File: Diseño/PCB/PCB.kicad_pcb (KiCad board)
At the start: 2 copper layers, 26 parts, among them J1 Bateria, P101 USB_C_Plug_USB2.0, Q101 SS8050, Q102 SS8050, U1 SDP31-500PA-TR-250PCS, U101 AMS1117-3.3, U102 CH340C, U2 SCD41-D-R2, U3 BME688

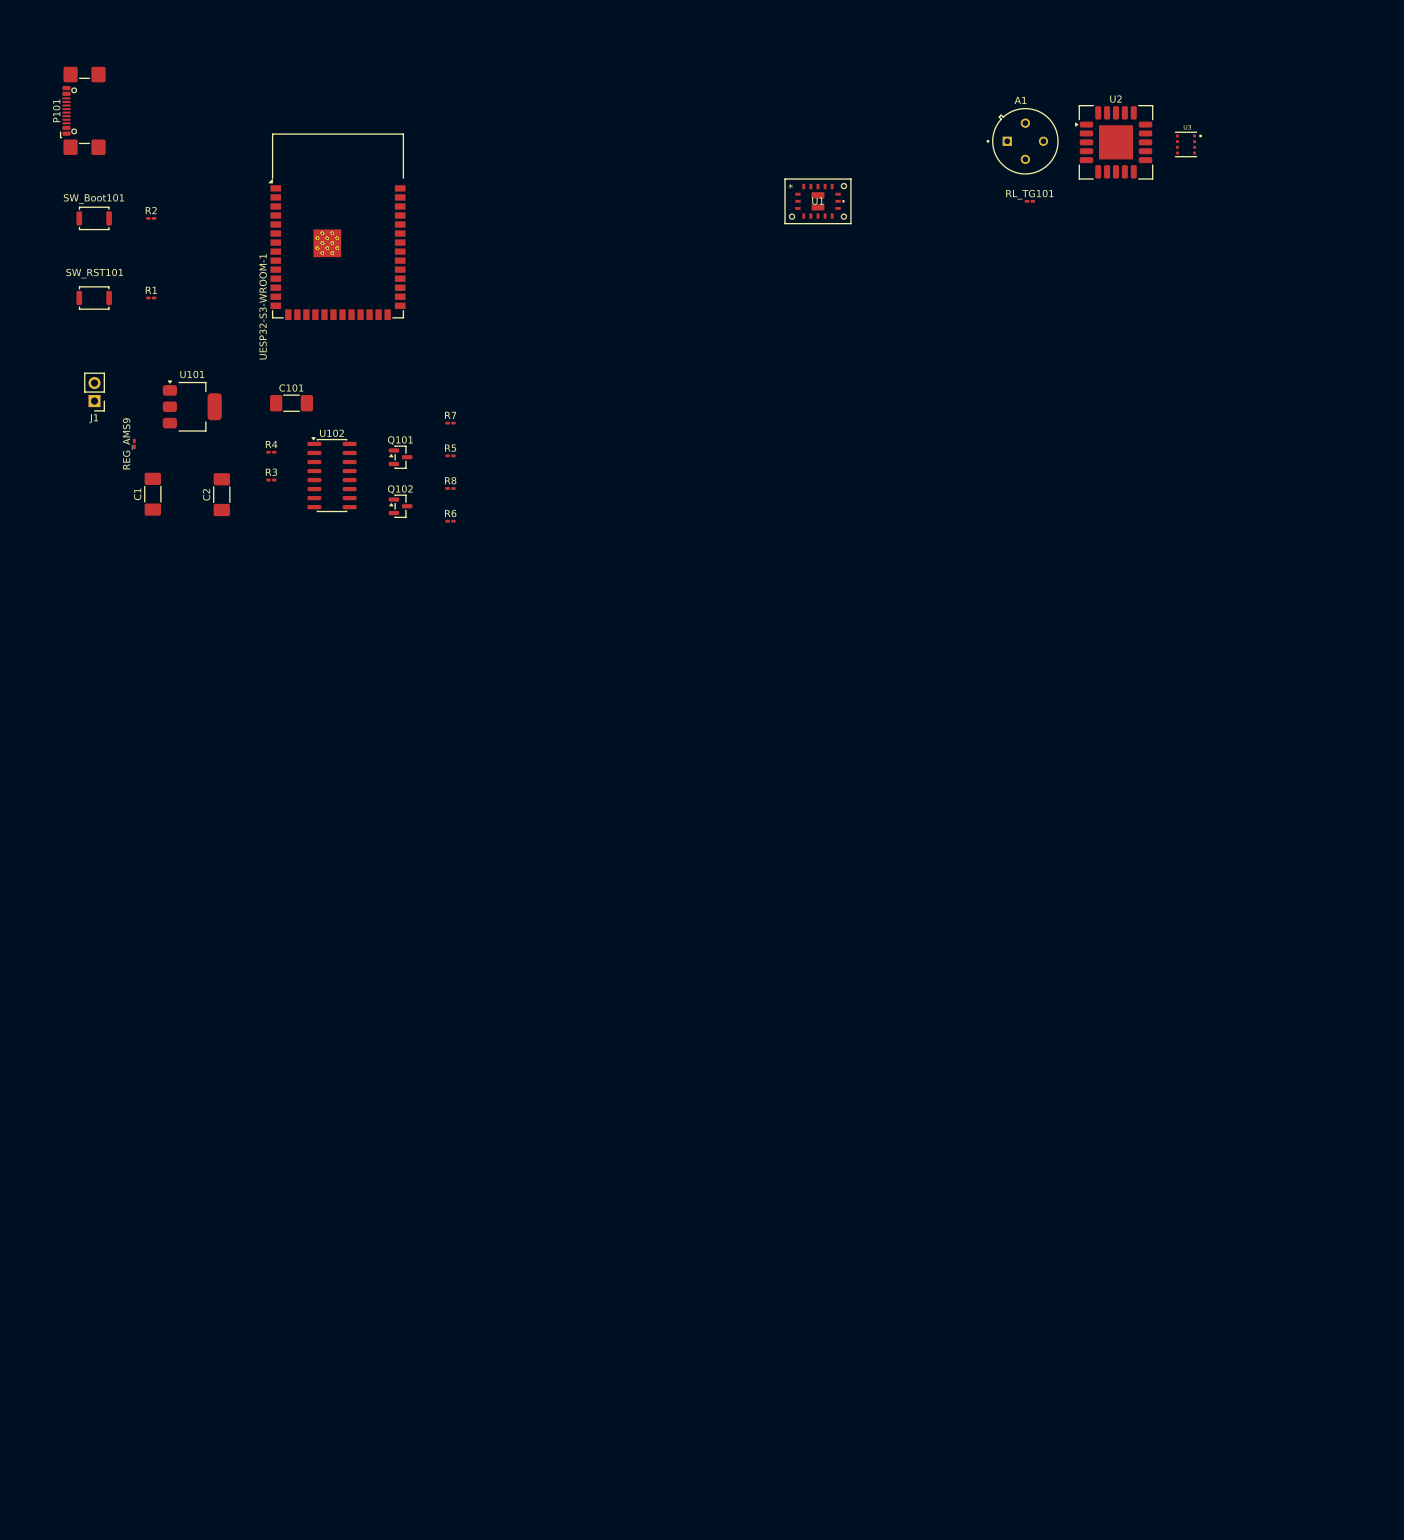
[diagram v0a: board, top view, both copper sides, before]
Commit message: Update
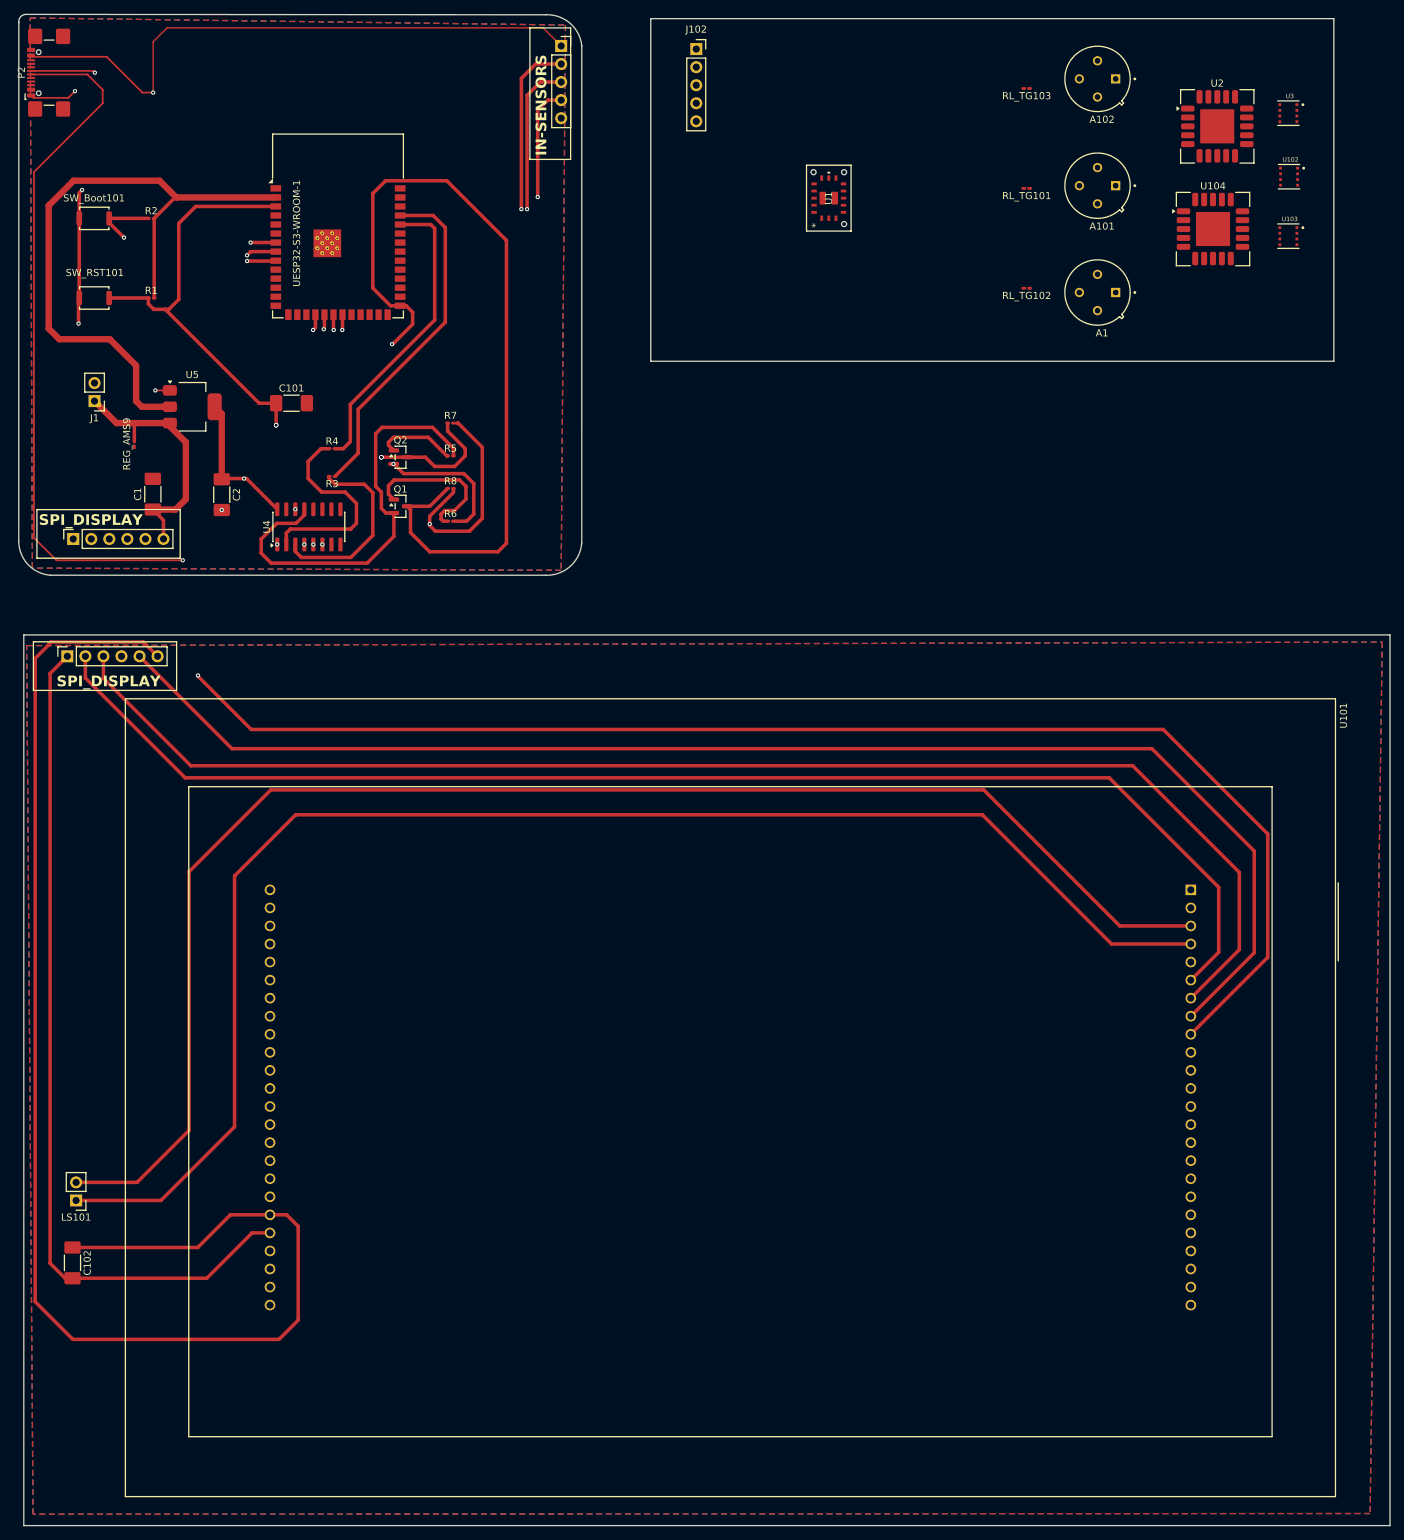
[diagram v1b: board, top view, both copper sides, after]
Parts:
- added A101: TGS2600, Propia:TO255P920H830-4, F.Cu at (207.8, 70.5)
- added A102: TGS2600, Propia:TO255P920H830-4, F.Cu at (207.8, 55.5)
- added C102: 100u, Capacitor_SMD:C_1808_4520Metric_Pad1.72x2.30mm_HandSolder, F.Cu at (63.5, 222.0)
- added G***: LOGO, Propia:LogoFiuba, B.Cu at (68.8, 52.0)
- added J101: Conn_01x05_Pin, Connector_PinSocket_2.54mm:PinSocket_1x05_P2.54mm_Vertical, F.Cu at (132.3, 50.8)
- added J102: Conn_01x05_Pin, Connector_PinSocket_2.54mm:PinSocket_1x05_P2.54mm_Vertical, F.Cu at (151.3, 51.3)
- added J103: Conn_01x06_Socket, Connector_PinSocket_2.54mm:PinSocket_1x06_P2.54mm_Vertical, F.Cu at (63.6, 120.2)
- added J104: Conn_01x06_Socket, Connector_PinSocket_2.54mm:PinSocket_1x06_P2.54mm_Vertical, F.Cu at (62.8, 136.7)
- added LS101: Speaker, Connector_PinHeader_2.54mm:PinHeader_1x02_P2.54mm_Vertical, F.Cu at (64.1, 213.3)
- added RL_TG102: 450, Resistor_SMD:R_0201_0603Metric_Pad0.64x0.40mm_HandSolder, F.Cu at (197.8, 84.9)
- added RL_TG103: 450, Resistor_SMD:R_0201_0603Metric_Pad0.64x0.40mm_HandSolder, F.Cu at (197.8, 56.8)
- added U101: EA_eDIPTFT70-ATP, Display:EA_eDIPTFT70-XXX, F.Cu at (220.9, 169.6)
- added U102: BME688, Propia:IC_BME688, F.Cu at (234.7, 69.2)
- added U103: BME688, Propia:IC_BME688, F.Cu at (234.6, 77.6)
- added U104: SCD41-D-R2, Sensor:Sensirion_SCD4x-1EP_10.1x10.1mm_P1.25mm_EP4.8x4.8mm, F.Cu at (224.0, 76.6)
- moved A1 23.6 mm to (207.8, 85.5), turned to 180 degrees
- moved U3 15.1 mm to (234.6, 60.3)
- moved U2 14.4 mm to (224.6, 62.1)
- moved R3 8.55 mm to (100.1, 111.4), turned to 180 degrees
- moved R4 8.55 mm to (100.1, 107.5)
- moved U4 7.93 mm to (96.8, 118.5), turned to 90 degrees
- moved P2 7.33 mm to (61.4, 54.6)
- moved RL_TG101 1.88 mm to (197.8, 70.9), turned to 180 degrees
- moved U1 1.59 mm to (169.9, 72.2), turned to 90 degrees
- turned C2 to -90 degrees
- renumbered P101 to P2, Q102 to Q1, Q101 to Q2, U102 to U4, U101 to U5
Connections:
- UESP32-S3-WROOM-1 pad 18: Analog_input -> SS
- UESP32-S3-WROOM-1 pad 19: unconnected-(UESP32-S3-WROOM-1-IO11-Pad19) -> MOSI
- UESP32-S3-WROOM-1 pad 20: unconnected-(UESP32-S3-WROOM-1-IO12-Pad20) -> CLK
- UESP32-S3-WROOM-1 pad 21: unconnected-(UESP32-S3-WROOM-1-IO13-Pad21) -> MISO
- UESP32-S3-WROOM-1 pad 7: unconnected-(UESP32-S3-WROOM-1-IO7-Pad7) -> Analog_input
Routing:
- net 5V: track 0.00 -> 369.6 mm, vias 0 -> 1
- net CLK: track 0.00 -> 255.8 mm, vias 0 -> 2
- net MISO: track 0.00 -> 247.2 mm, vias 0 -> 1
- net MOSI: track 0.00 -> 246.2 mm, vias 0 -> 1
- net SS: track 0.00 -> 240.9 mm, vias 0 -> 1
- net Net-(U101-SND+): track 0.00 -> 208.9 mm
- net Net-(U101-SND-): track 0.00 -> 207.5 mm
- net GND: track 0.00 -> 192.0 mm, vias 0 -> 6
- net 3.3V: track 0.00 -> 175.7 mm, vias 0 -> 3
- net Boot: track 0.00 -> 170.4 mm, vias 0 -> 2
- net D+: track 0.00 -> 119.5 mm, vias 0 -> 2
- net D-: track 0.00 -> 112.7 mm, vias 0 -> 2
- net EN: track 0.00 -> 96.3 mm, vias 0 -> 6
- net SCL: track 0.00 -> 71.1 mm, vias 0 -> 2
- net SDA: track 0.00 -> 68.7 mm, vias 0 -> 2
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- added copper zone on B.Cu, net GND
- added copper zone on F.Cu, net GND
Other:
- board outline added: 192.9 x 212.6 mm
- copper layers 2 -> 6
- board text added: "IN-SENSORS"
- board text added: "SPI_DISPLAY"
